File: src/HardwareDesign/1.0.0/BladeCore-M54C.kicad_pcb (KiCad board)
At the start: 6 copper layers, 29 x 80.6 mm, 152 parts, among them IC1 RP2354B, IC2 AT24C256C-XHL-T, IC29 TCAN1044AVDRBRQ1, IC3 W25Q128JVPIQ, IC4 MCP6001RT, IC5 LM4040B30FTA, IC6 MCP2515T-I/ML, IC7 TPS74801DRCT, IC8 SN74LVC1G97QDCKRQ1, IC9 FSUSB42MUX, J1 MDT320M03001, J2 SM03B-SRSS-TB, J3 USB-TYPE-C-018, SW1 B3U-1000P, SW2 B3U-1000P, X1 12MHz 10pF, X2 16MHz 8pF

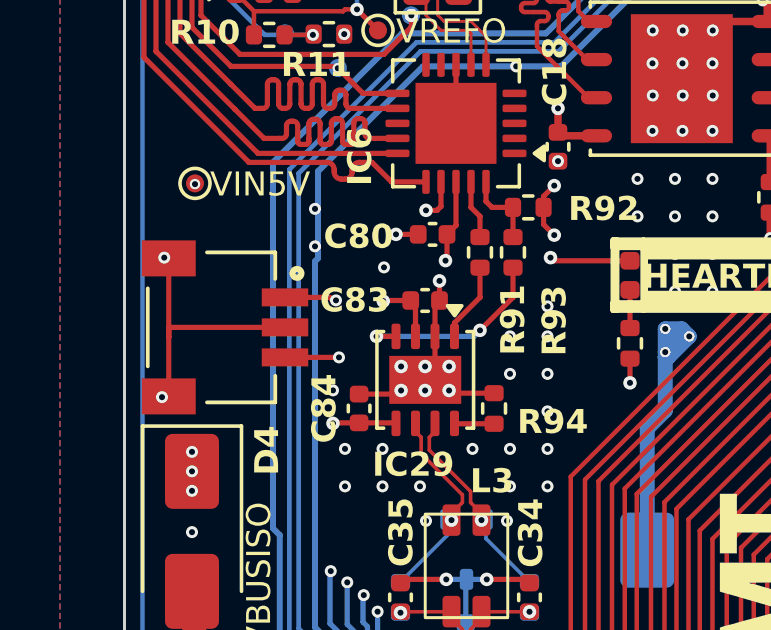
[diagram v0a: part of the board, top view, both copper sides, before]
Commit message: update generator
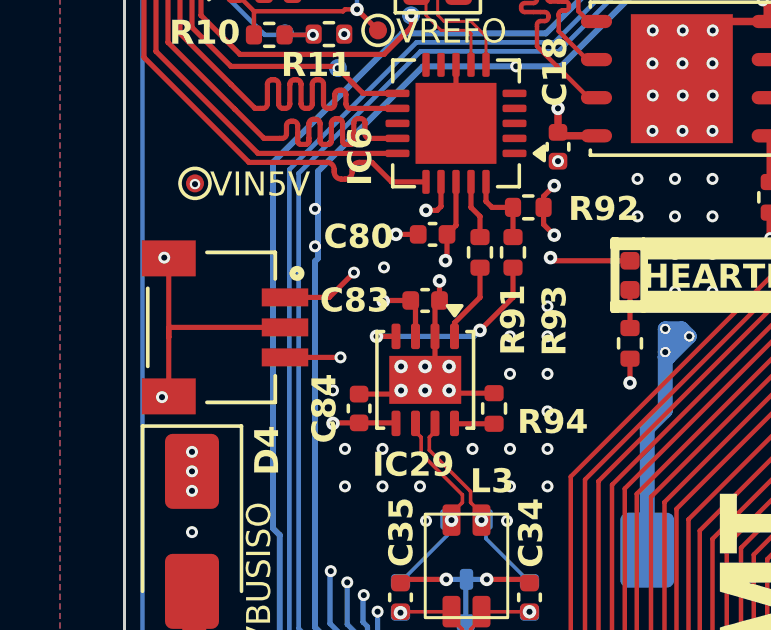
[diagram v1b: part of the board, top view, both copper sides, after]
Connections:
- J2 pad 1: /Project Architecture/Microcontroller Peripherals/SWDIO -> /Project Architecture/Microcontroller Peripherals/SWCLK
- J2 pad 3: /Project Architecture/Microcontroller Peripherals/SWCLK -> /Project Architecture/Microcontroller Peripherals/SWDIO
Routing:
- net /Project Architecture/Microcontroller Peripherals/SWCLK: track 40.9 -> 38.7 mm
- net /Project Architecture/Microcontroller Peripherals/SWDIO: track 40.2 -> 42.2 mm
